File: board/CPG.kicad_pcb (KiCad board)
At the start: 2 copper layers, 150 x 48 mm, 65 parts, among them J1 1, J2 2, J3 3, J4 4, J5 5, U1 PAN2110P0AA, U2 HLK-PM03, U3 PY32F030K1xTx, U4 MOC306XMS, U5 MOC306XMS, U6 MOC306XMS, U7 MOC306XMS, U8 MOC306XMS, X1 SWD, Y1 16MHz

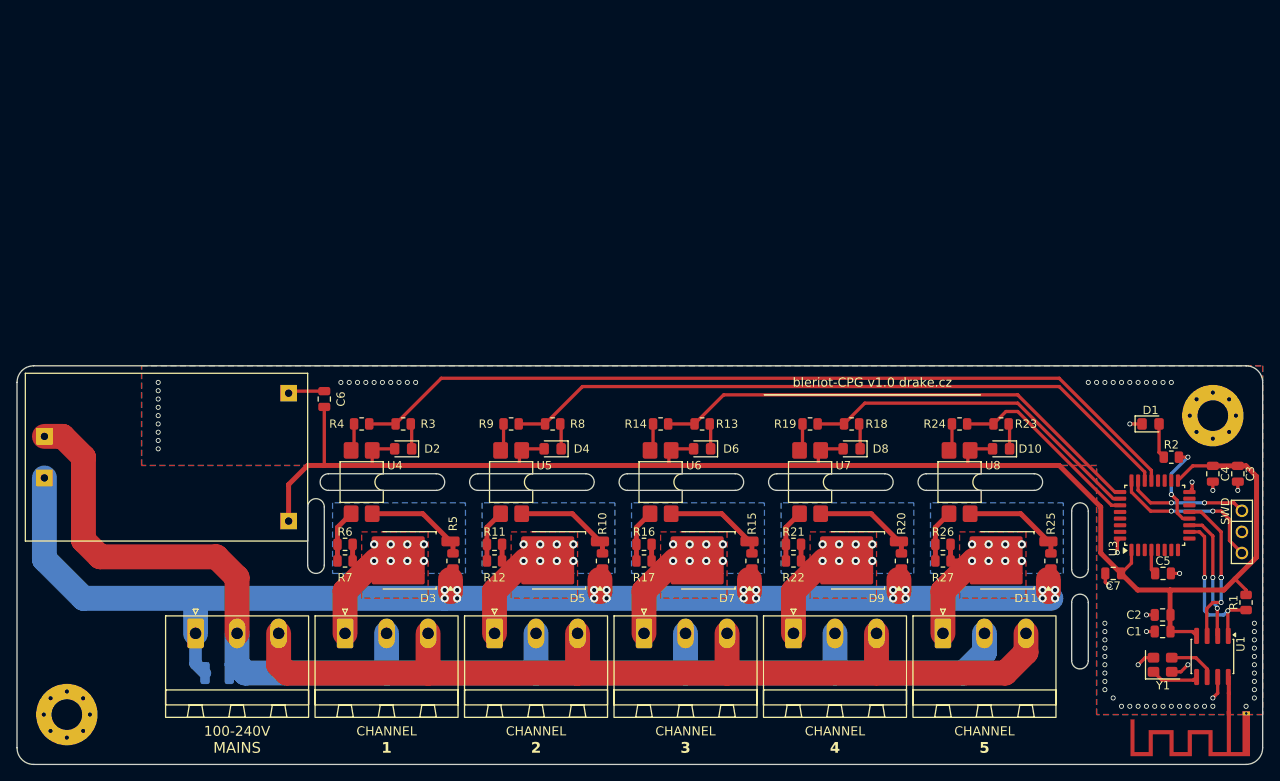
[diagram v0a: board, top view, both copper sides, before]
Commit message: WIP
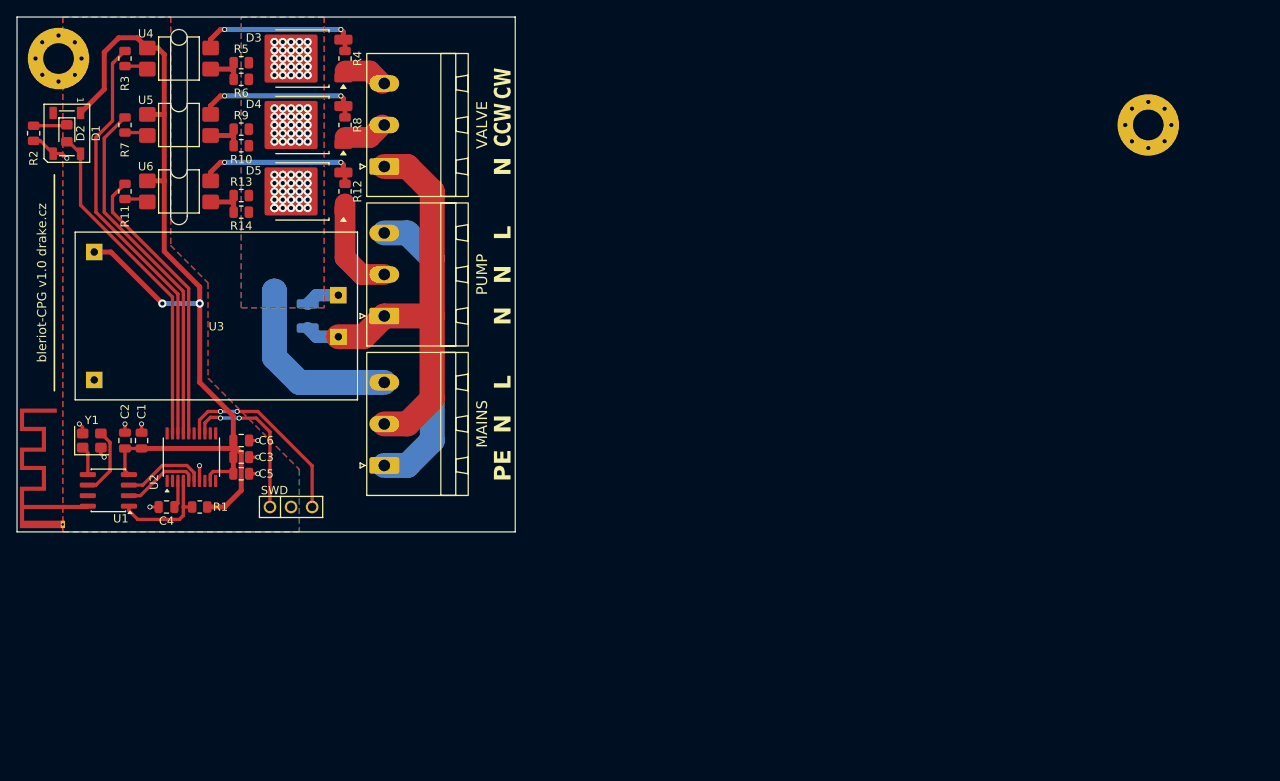
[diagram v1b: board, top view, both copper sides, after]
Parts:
- removed C7: 100n, Capacitor_SMD:C_0805_2012Metric
- removed D10, D6, D8: LED, LED_SMD:LED_0805_2012Metric_Pad1.15x1.40mm_HandSolder
- removed D11, D7, D9: BTA08S-600CW, Package_TO_SOT_SMD:TO-252-2
- removed IN1: MAINS, Connector_Phoenix_MSTB:PhoenixContact_MSTBA_2,5_3-G_1x03_P5.00mm_Horizontal
- removed J4: 4, Connector_Phoenix_MSTB:PhoenixContact_MSTBA_2,5_3-G_1x03_P5.00mm_Horizontal
- removed J5: 5, Connector_Phoenix_MSTB:PhoenixContact_MSTBA_2,5_3-G_1x03_P5.00mm_Horizontal
- removed R15, R16, R17, R20, R21, R22, R25, R26, R27: 680R, Resistor_SMD:R_0805_2012Metric
- removed R18, R23: 330R, Resistor_SMD:R_0805_2012Metric
- removed R19, R24: 270R, Resistor_SMD:R_0805_2012Metric
- removed U7, U8: MOC306XMS, Package_DIP:SMDIP-4_W7.62mm
- D1: value LED -> WS2812B; footprint LED_SMD:LED_0805_2012Metric_Pad1.15x1.40mm_HandSolder -> LED_SMD:LED_WS2812B_PLCC4_5.0x5.0mm_P3.2mm
- D4: value LED -> BTA08S-600CW; footprint LED_SMD:LED_0805_2012Metric_Pad1.15x1.40mm_HandSolder -> Package_TO_SOT_SMD:TO-252-2
- J1: value 1 -> MAINS
- J2: value 2 -> VALVE
- J3: value 3 -> PUMP
- R11, R7: value 680R -> 270R
- R13, R8: value 330R -> 680R
- R14, R4, R9: value 270R -> 680R
- R3: value 330R -> 270R
- U2: value HLK-PM03 -> PY32F030F1xPx; footprint Drake:HLK-PM01 -> Package_SO:TSSOP-20_4.4x6.5mm_P0.65mm
- U3: value PY32F030K1xTx -> HLK-PM03; footprint Package_QFP:LQFP-32_7x7mm_P0.8mm -> Drake:HLK-PM01
- moved A1 142.6 mm to (85.5, 106.0), turned to 90 degrees
- moved R2 142.4 mm to (82.0, 61.0), turned to 90 degrees
- moved D1 135.1 mm to (86.0, 61.0), turned to -90 degrees
- moved U1 134.4 mm to (91.0, 104.0), turned to 180 degrees
- moved Y1 131.7 mm to (89.0, 98.0)
- moved C2 126.7 mm to (93.0, 98.0), turned to 90 degrees
- moved R1 126.5 mm to (102.0, 106.0), turned to 0 degrees
- moved C4 126.1 mm to (98.0, 106.0), turned to 180 degrees
- moved C1 125.1 mm to (95.0, 98.0), turned to 90 degrees
- moved C3 120.0 mm to (107.0, 100.0), turned to 0 degrees
- moved U3 115.5 mm to (104.0, 83.0), turned to 180 degrees
- moved X1 114.5 mm to (113.0, 106.0), turned to 0 degrees
- moved C5 111.6 mm to (107.0, 102.0)
- moved H1 79.0 mm to (85.0, 52.0)
- moved U6 67.7 mm to (99.5, 68.0), turned to 0 degrees
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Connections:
- C4 pad 1: +3V3 -> Net-(U2-PF2-NRST)
- C5 pad 1: Net-(U3-PF2-NRST) -> +3V3
- D1 pad 1: GND -> +3V3
- D1 pad 2: Net-(D1-A) -> unconnected-(D1-DOUT-Pad2)
- D2 pad 2: +3V3 -> /LED
- D3 pad 1: MAINS-L -> /valve-cw/OUT
- D3 pad 2: Net-(D3-A2) -> MAINS-L
- D4 pad 1: Net-(D4-K) -> /valve-ccw/OUT
- D4 pad 2: +3V3 -> MAINS-L
- D5 pad 1: MAINS-L -> /pump/OUT
- D5 pad 2: Net-(D5-A2) -> MAINS-L
- J1 pad 1: Net-(D3-A2) -> MAINS-PE
- J1 pad 3: MAINS-PE -> MAINS-L
- J2 pad 1: Net-(D5-A2) -> MAINS-N
- J2 pad 2: MAINS-N -> /valve-ccw/OUT
- J2 pad 3: MAINS-PE -> /valve-cw/OUT
- J3 pad 1: Net-(D7-A2) -> MAINS-N
- J3 pad 2: MAINS-N -> /pump/OUT
- R10 pad 1: Net-(D5-G) -> MAINS-L
- R10 pad 2: MAINS-L -> Net-(R10-Pad2)
- R11 pad 1: Net-(R11-Pad1) -> /PUMP
- R11 pad 2: Net-(D5-A2) -> Net-(R11-Pad2)
- R12 pad 1: Net-(D5-A2) -> Net-(D5-G)
- R12 pad 2: Net-(R11-Pad1) -> /pump/OUT
- R13 pad 1: ~{CH3} -> Net-(R13-Pad1)
- R13 pad 2: Net-(D6-K) -> MAINS-L
- R14 pad 1: ~{CH3} -> MAINS-L
- R14 pad 2: Net-(R14-Pad2) -> Net-(R13-Pad1)
- R2 pad 1: Net-(D1-A) -> GND
- R2 pad 2: /LED -> Net-(D2-K)
- R3 pad 1: ~{CH1} -> /VALVE_CW
- R3 pad 2: Net-(D2-K) -> Net-(R3-Pad2)
- R4 pad 1: ~{CH1} -> Net-(D3-G)
- R4 pad 2: Net-(R4-Pad2) -> /valve-cw/OUT
- R5 pad 1: Net-(D3-G) -> Net-(R5-Pad1)
- R6 pad 1: Net-(R6-Pad1) -> MAINS-L
- R6 pad 2: Net-(D3-A2) -> Net-(R5-Pad1)
- R7 pad 1: Net-(D3-A2) -> /VALVE_CCW
- R7 pad 2: Net-(R6-Pad1) -> Net-(R7-Pad2)
- R8 pad 1: ~{CH2} -> Net-(D4-G)
- R8 pad 2: Net-(D4-K) -> /valve-ccw/OUT
- R9 pad 1: ~{CH2} -> Net-(R10-Pad2)
- R9 pad 2: Net-(R9-Pad2) -> MAINS-L
- U2 pad 1: MAINS-N -> unconnected-(U2-PF0-OSCIN-Pad1)
- U2 pad 2: MAINS-L -> unconnected-(U2-PF1-OSCOUT-Pad2)
- U2 pad 3: GND -> Net-(U2-PF2-NRST)
- U2 pad 4: +3V3 -> /~{RF_CS}
- U3 pad 1: +3V3 -> MAINS-N
- U3 pad 2: unconnected-(U3-PF0-OSCIN-Pad2) -> MAINS-L
- U3 pad 3: unconnected-(U3-PF1-OSCOUT-Pad3) -> GND
- U3 pad 4: Net-(U3-PF2-NRST) -> +3V3
- U4 pad 2: Net-(R4-Pad2) -> Net-(R3-Pad2)
- U4 pad 3: Net-(R6-Pad1) -> Net-(R5-Pad1)
- U5 pad 2: Net-(R9-Pad2) -> Net-(R7-Pad2)
- U5 pad 3: Net-(R11-Pad1) -> Net-(R10-Pad2)
- U5 pad 4: Net-(D5-G) -> Net-(D4-G)
- U6 pad 2: Net-(R14-Pad2) -> Net-(R11-Pad2)
- U6 pad 3: Net-(R16-Pad1) -> Net-(R13-Pad1)
- U6 pad 4: Net-(D7-G) -> Net-(D5-G)
- X1 pad 1: Net-(U3-PA13-SWD) -> Net-(U2-PA11)
- X1 pad 3: Net-(U3-PA14-SWC) -> Net-(U2-PA13)
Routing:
- net MAINS-L: track 153.9 -> 29.6 mm, vias 20 -> 76
- net MAINS-N: track 159.4 -> 55.5 mm, vias 0 -> 1
- net ~{CH1}: track 102.3 -> 0.00 mm
- net ~{CH2}: track 82.5 -> 0.00 mm
- net MAINS-PE: track 116.6 -> 36.0 mm
- net +3V3: track 196.4 -> 121.5 mm, vias 0 -> 2
- net ~{CH3}: track 60.7 -> 0.00 mm
- net /VALVE_CW: track 0.00 -> 51.6 mm
- net /VALVE_CCW: track 0.00 -> 43.0 mm
- net ~{CH4}: track 42.2 -> 0.00 mm
- net /PUMP: track 0.00 -> 34.5 mm
- net /LED: track 10.7 -> 40.5 mm, vias 2 -> 0
- net ~{CH5}: track 23.7 -> 0.00 mm
- net Net-(U2-PA13): track 0.00 -> 23.3 mm, vias 0 -> 2
- net Net-(D4-G): track 0.00 -> 20.0 mm, vias 0 -> 2
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- added copper zone on B.Cu, net MAINS-L
- added copper zone on F.Cu, net MAINS-L
- removed copper zone on B.Cu, net Net-(D11-A2)
- removed copper zone on F.Cu, net Net-(D11-A2)
- removed copper zone on F.Cu, net Net-(D3-A2)
- removed copper zone on F.Cu, net Net-(D5-A2)
- removed copper zone on F.Cu, net Net-(D7-A2)
- removed copper zone on F.Cu, net Net-(D9-A2)
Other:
- board size 150 x 48 mm -> 60 x 62 mm
- board text added: "CCW"
- board text added: "CW"
- board text added: "L"
- board text added: "N"
- board text added: "PE"
- board text added: "PUMP"
- board text added: "VALVE"
- board text removed: "100-240V"
- board text removed: "CHANNEL"
